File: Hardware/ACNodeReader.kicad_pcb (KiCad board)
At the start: 2 copper layers, 50 x 50 mm, 29 parts, among them J1 8P8C, J2 AVR-ISP-6, J3 Conn_01x04_Female, J5 Conn_01x04_Female, SW2 SW_Push, U1 L78L05_SOT89, U2 ATmega88PB-AU, U3 ISL8489EIBZ, U4 SI7060-B-00-IV, Y1 Crystal_GND24

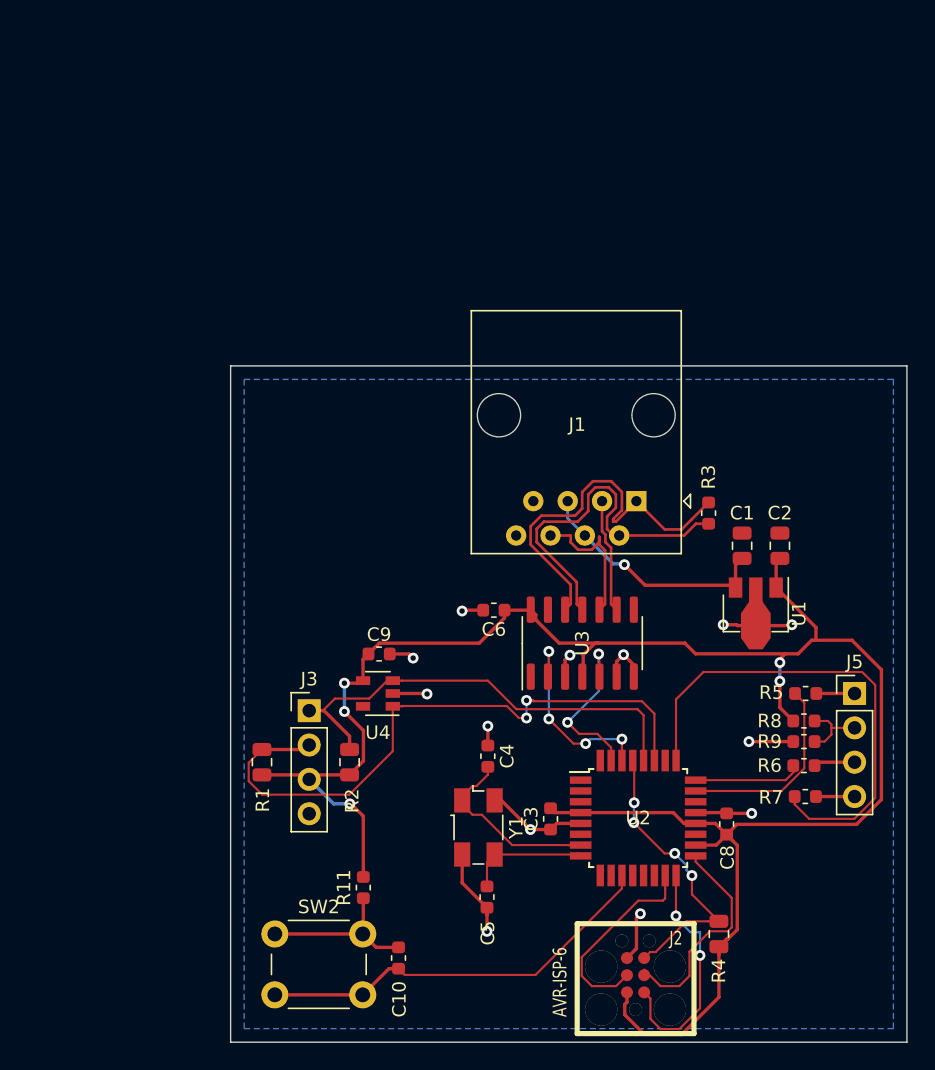
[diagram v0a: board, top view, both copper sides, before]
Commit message: New, smaller, better PCB design
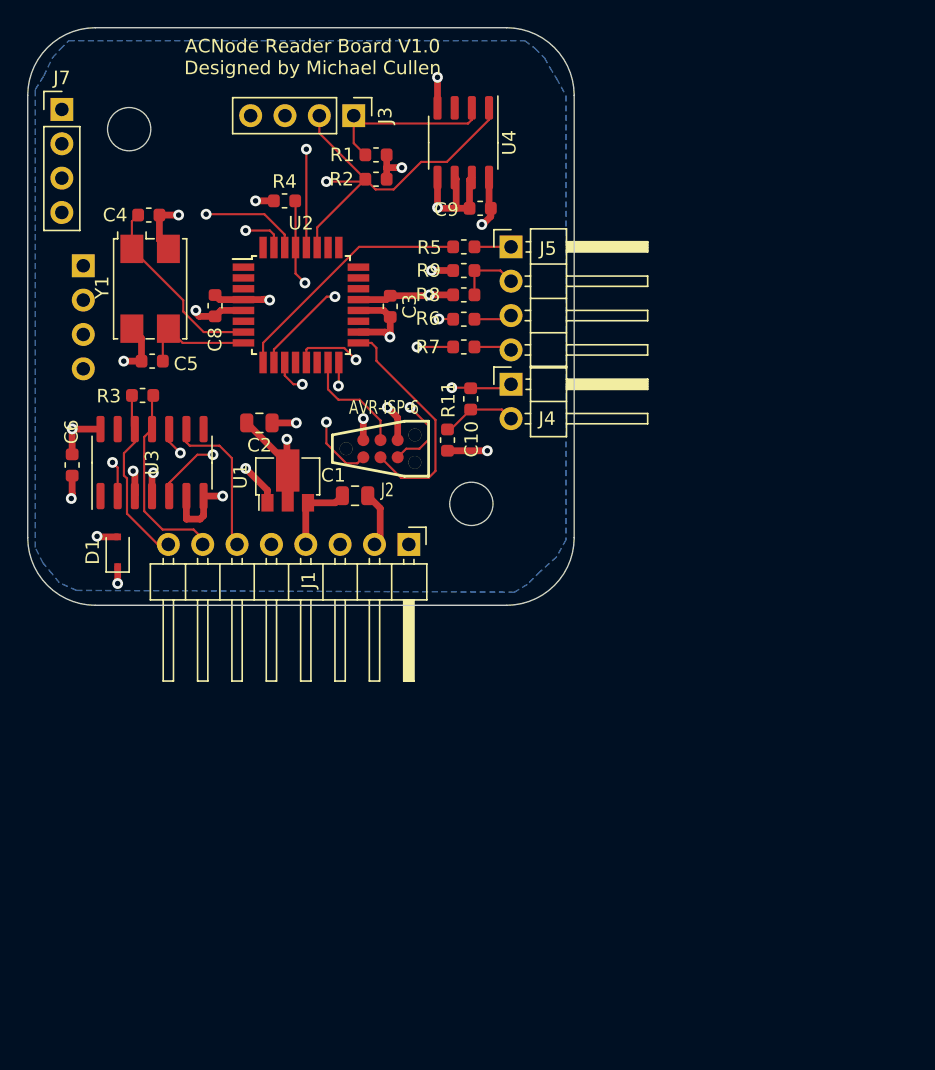
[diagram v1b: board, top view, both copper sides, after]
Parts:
- removed SW2: SW_Push, Button_Switch_THT:SW_PUSH_6mm
- added D1: D_Zener, Diode_SMD:D_SOD-323F, F.Cu at (116.6, 98.7)
- added H1: MountingHole, MountingHole:MountingHole_3.2mm_M3_DIN965, F.Cu at (117.5, 67.5)
- added H2: MountingHole, MountingHole:MountingHole_3.2mm_M3_DIN965, F.Cu at (142.8, 95.2)
- added J4: Conn_01x02_Male, Connector_PinHeader_2.54mm:PinHeader_1x02_P2.54mm_Horizontal, F.Cu at (145.7, 86.4)
- added J6: Conn_01x04_Male, Connector_PinHeader_2.54mm:PinHeader_1x04_P2.54mm_Horizontal, B.Cu at (114.1, 77.6)
- added J7: Conn_01x04_Male, Connector_PinHeader_2.54mm:PinHeader_1x04_P2.54mm_Vertical, F.Cu at (112.5, 66.0)
- J1: value 8P8C -> Conn_01x08_Male; footprint Connector_RJ:RJ45_Amphenol_54602-x08_Horizontal -> Connector_PinHeader_2.54mm:PinHeader_1x08_P2.54mm_Horizontal
- J2: footprint Tag-Connect:TC2030-MCP -> Tag-Connect:TC2030-MCP-NL
- J5: footprint Connector_PinHeader_2.54mm:PinHeader_1x04_P2.54mm_Vertical -> Connector_PinHeader_2.54mm:PinHeader_1x04_P2.54mm_Horizontal
- R1, R2, R4: footprint Resistor_SMD:R_0805_2012Metric -> Resistor_SMD:R_0603_1608Metric
- U4: value SI7060-B-00-IV -> LM75C; footprint Package_TO_SOT_SMD:SOT-23-5 -> Package_SO:SO-8_3.9x4.9mm_P1.27mm
- Y1: footprint Crystal:Crystal_SMD_Abracon_ABM3B-4Pin_5.0x3.2mm -> Crystal:Crystal_SMD_7050-4Pin_7.0x5.0mm
- moved R4 63.0 mm to (129.0, 72.8), turned to 0 degrees
- moved C8 53.8 mm to (123.8, 80.5), turned to 270 degrees
- moved C4 47.2 mm to (119.0, 73.8), turned to 180 degrees
- moved C5 46.7 mm to (119.2, 84.7), turned to 0 degrees
- moved J2 46.7 mm to (133.5, 91.1), turned to 0 degrees
- moved Y1 46.6 mm to (119.0, 79.3)
- moved R1 45.7 mm to (135.8, 69.4), turned to 0 degrees
- moved U2 45.4 mm to (130.2, 80.5)
- moved J3 44.1 mm to (134.1, 66.5), turned to 270 degrees
- moved R2 43.1 mm to (135.8, 71.2), turned to 0 degrees
- moved R9 43.0 mm to (142.2, 78.0)
- moved R3 42.7 mm to (118.5, 87.2), turned to 0 degrees
- moved R7 41.7 mm to (142.2, 83.6)
- moved C10 41.7 mm to (142.7, 87.4), turned to 270 degrees
- moved J5 41.7 mm to (145.7, 76.2)
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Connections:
- J1 pad 1: /RX+ -> GND
- J1 pad 2: /RX- -> GND
- J1 pad 3: /TX+ -> /TX-
- J1 pad 6: /TX- -> /TX+
- J1 pad 7: GND -> /RX-
- J1 pad 8: GND -> /RX+
- R1 pad 1: i2c_SDA -> i2c_SCL
- R2 pad 1: i2c_SCL -> i2c_SDA
- R5 pad 2: Net-(R5-Pad2) -> /LED1
- R6 pad 2: Net-(R6-Pad2) -> /LED2
- R7 pad 2: Net-(R7-Pad2) -> /LED3
- R8 pad 2: +5V -> GND
- R9 pad 1: GND -> +5V
- U2 pad 10: Net-(U2-Pad10) -> /LED2
- U2 pad 13: Net-(U2-Pad13) -> /LED3
- U2 pad 23: Net-(R5-Pad2) -> Net-(U2-Pad23)
- U2 pad 24: Net-(R6-Pad2) -> Net-(U2-Pad24)
- U2 pad 25: Net-(R7-Pad2) -> Net-(U2-Pad25)
- U2 pad 9: Net-(U2-Pad9) -> /LED1
- U4 pad 2: GND -> i2c_SCL
- U4 pad 3: i2c_SCL -> Net-(U4-Pad3)
- U4 pad 4: +5V -> GND
- U4 pad 5: Net-(U4-Pad5) -> GND
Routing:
- net Net-(R7-Pad2): track 36.5 -> 0.00 mm
- net /uC_TX: track 12.7 -> 42.0 mm
- net /uC_RX: track 14.8 -> 33.7 mm, vias 4 -> 2
- net /LED1: track 0.00 -> 18.7 mm
- net +5V: track 148.7 -> 166.2 mm, vias 5 -> 12
- net /LED2: track 0.00 -> 16.8 mm, vias 0 -> 2
- net GND: track 47.1 -> 62.4 mm, vias 13 -> 12
- net /RX+: track 28.6 -> 13.7 mm
- net Net-(R5-Pad2): track 14.5 -> 0.00 mm
- net /LED3: track 0.00 -> 12.9 mm, vias 0 -> 2
- net /RX-: track 26.5 -> 14.6 mm
- net i2c_SCL: track 34.8 -> 44.2 mm, vias 0 -> 1
- net Net-(C10-Pad1): track 30.3 -> 21.2 mm, vias 0 -> 2
- net Net-(R6-Pad2): track 8.27 -> 0.00 mm
- net Net-(J2-Pad1): track 17.7 -> 9.89 mm
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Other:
- board size 50 x 50 mm -> 40.4 x 42.7 mm
- copper layers 2 -> 4
- net class Power: trace_width 0.25 -> 0.5
- board text added: "+5V"
- board text added: "2020-08-27"
- board text added: "ACNode Reader Board V1.0 Designed by Michael Cullen"
- board text added: "Blue"
- board text added: "Blue/White"
- board text added: "Brown"
- board text added: "Brown/White"
- board text added: "Common"
- board text added: "Display?"
- board text added: "Fit R8 for common anode Fit R9 for common cathode Fit both for exciting times (briefly)"
- board text added: "GND"
- board text added: "Gr/Wh"
- board text added: "Green"
- board text added: "LED"
- board text added: "O/W"
- board text added: "Orange"
- board text added: "PN532 Goes Here"
- board text added: "RX"
- board text added: "Red"
- board text added: "Switch"
- board text added: "TX"
- board text added: "To ACNode"
- board text added: "To ACNode (Alternative)"
